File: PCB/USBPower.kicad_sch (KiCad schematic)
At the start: 57 parts, among them Q10 PMOS, Q11 PMOS, Q12 PMOS, Q13 PMOS, Q2 PMOS, Q3 PMOS, Q4 PMOS, Q5 PMOS, Q6 PMOS, Q7 PMOS, Q8 PMOS, Q9 PMOS, U12 LM338T/NOPB, U13 LM338T/NOPB, U14 LM338T/NOPB, U16 LM338T/NOPB, U17 LM338T/NOPB, U18 LM338T/NOPB, U19 LM338T/NOPB, U20 LM338T/NOPB, U21 LM338T/NOPB, U22 LM338T/NOPB, U23 LM338T/NOPB

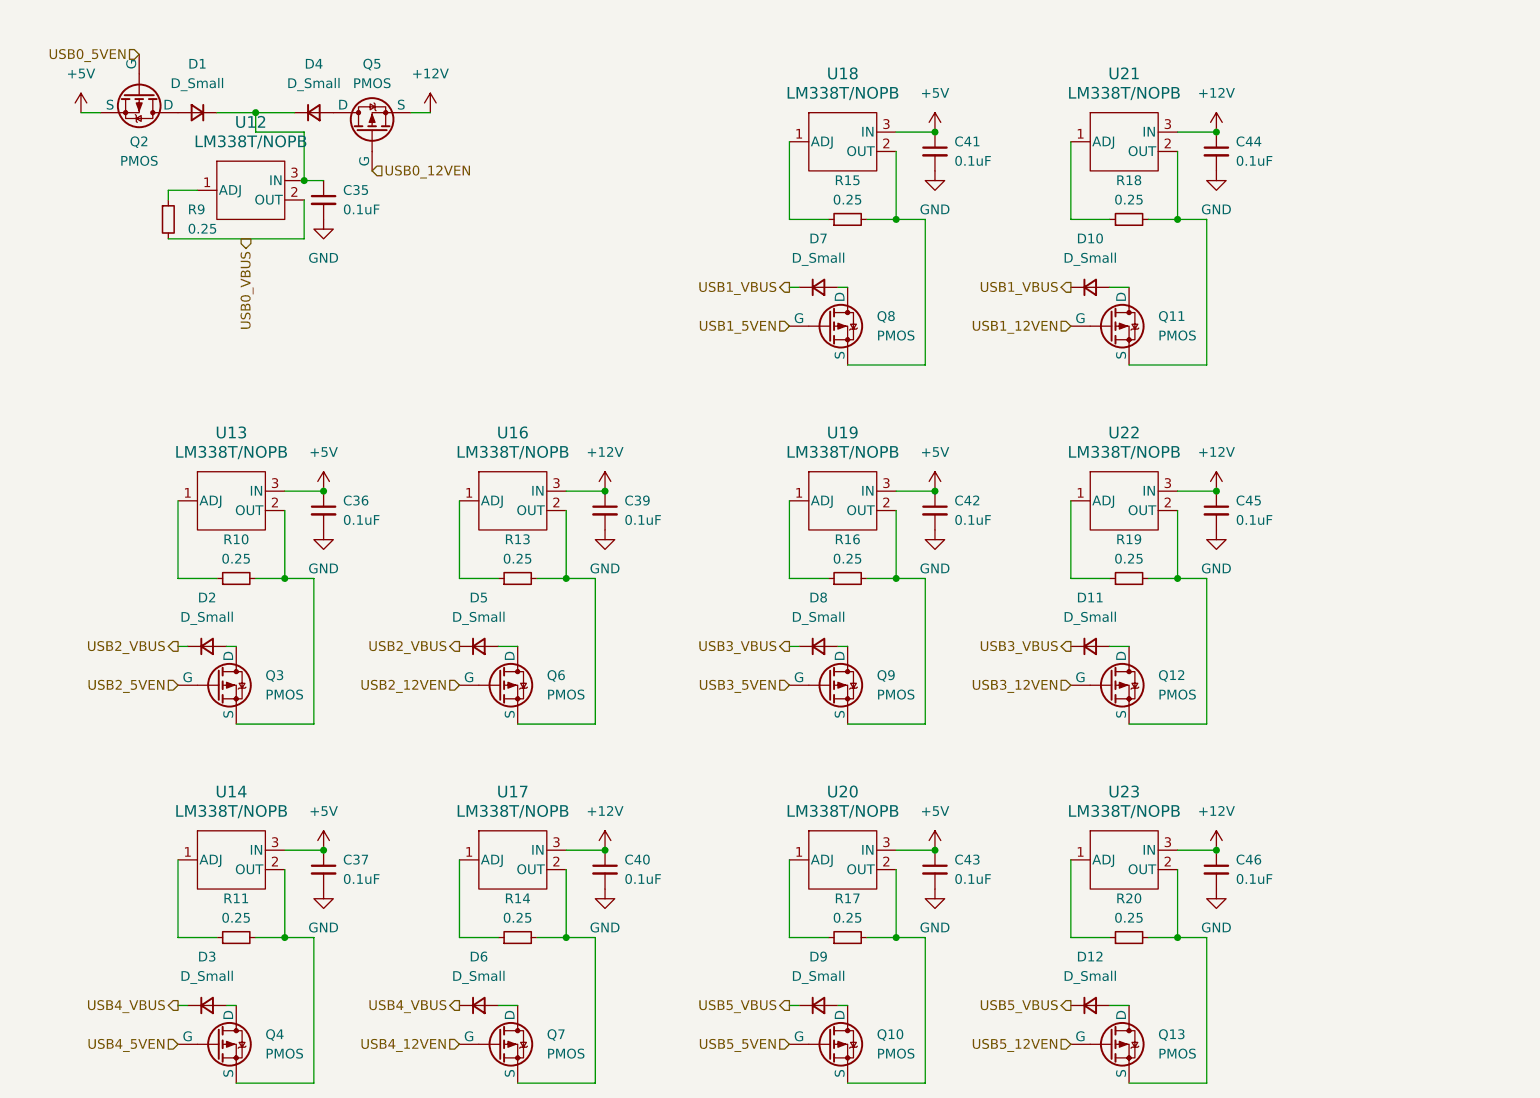
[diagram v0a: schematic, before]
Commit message: confused now
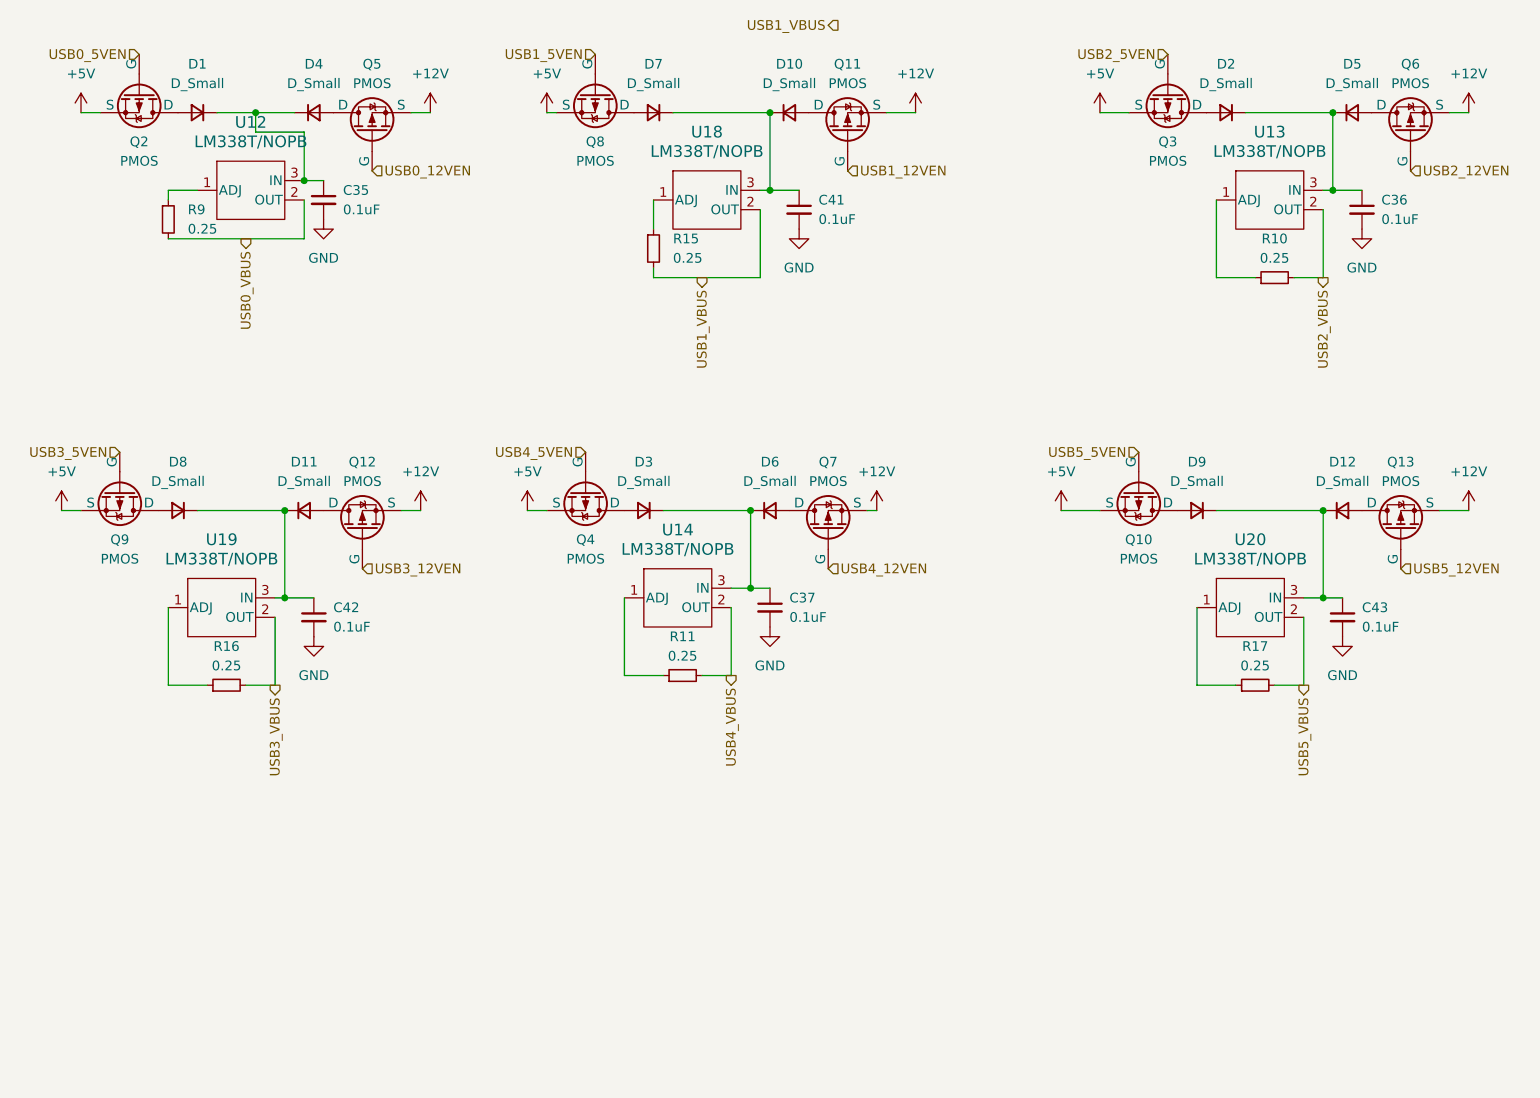
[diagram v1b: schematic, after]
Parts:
- removed C39, C40, C44, C45, C46: 0.1uF, Capacitor_SMD:C_0603_1608Metric_Pad1.08x0.95mm_HandSolder, symbol Device:C_Small
- removed R13, R14, R18, R19, R20: 0.25, Resistor_SMD:R_0603_1608Metric_Pad0.98x0.95mm_HandSolder, symbol Device:R_Small
- removed U16, U17, U21, U22, U23: LM338T/NOPB, LM338:T03B_TEX, symbol LM338:LM338T_NOPB
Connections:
- net +12V: now also Q11.3 (S), Q12.3 (S), Q13.3 (S), Q6.3 (S), Q7.3 (S)
- net +5V: now also Q10.3 (S), Q3.3 (S), Q4.3 (S), Q8.3 (S), Q9.3 (S); no longer C36.1, C37.1, C41.1, C42.1, C43.1, U13.3 (IN), U14.3 (IN), U18.3 (IN), U19.3 (IN), U20.3 (IN)
- net USB1_VBUS: now also R15.2, U18.2 (OUT); no longer D10.1 (K), D7.1 (K)
- net USB2_VBUS: now also R10.2, U13.2 (OUT); no longer D2.1 (K), D5.1 (K)
- net USB3_VBUS: now also R16.2, U19.2 (OUT); no longer D11.1 (K), D8.1 (K)
- net USB4_VBUS: now also R11.2, U14.2 (OUT); no longer D3.1 (K), D6.1 (K)
- net USB5_VBUS: now also R17.2, U20.2 (OUT); no longer D12.1 (K), D9.1 (K)
- new net: C37.1, D3.1 (K), D6.1 (K), U14.3 (IN)
- new net: C42.1, D11.1 (K), D8.1 (K), U19.3 (IN)
- new net: C43.1, D12.1 (K), D9.1 (K), U20.3 (IN)
- new net: C36.1, D2.1 (K), D5.1 (K), U13.3 (IN)
- new net: C41.1, D10.1 (K), D7.1 (K), U18.3 (IN)
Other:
- moved on the sheet: C36, C37, C41, C42, C43, D10, D11, D12, D2, D3, D5, D6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
